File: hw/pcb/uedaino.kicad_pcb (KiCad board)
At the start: 2 copper layers, 34 parts, among them IC1 ATMEGA328P-A, P1 CN_PWR, P2 CN_UART, P3 CN_HEADER1, P4 CN_I2C, P5 CN_HEADER2, P6 CN_ICSP, SW1 SW_PUSH, U1 AP1117, Y1 16MHz

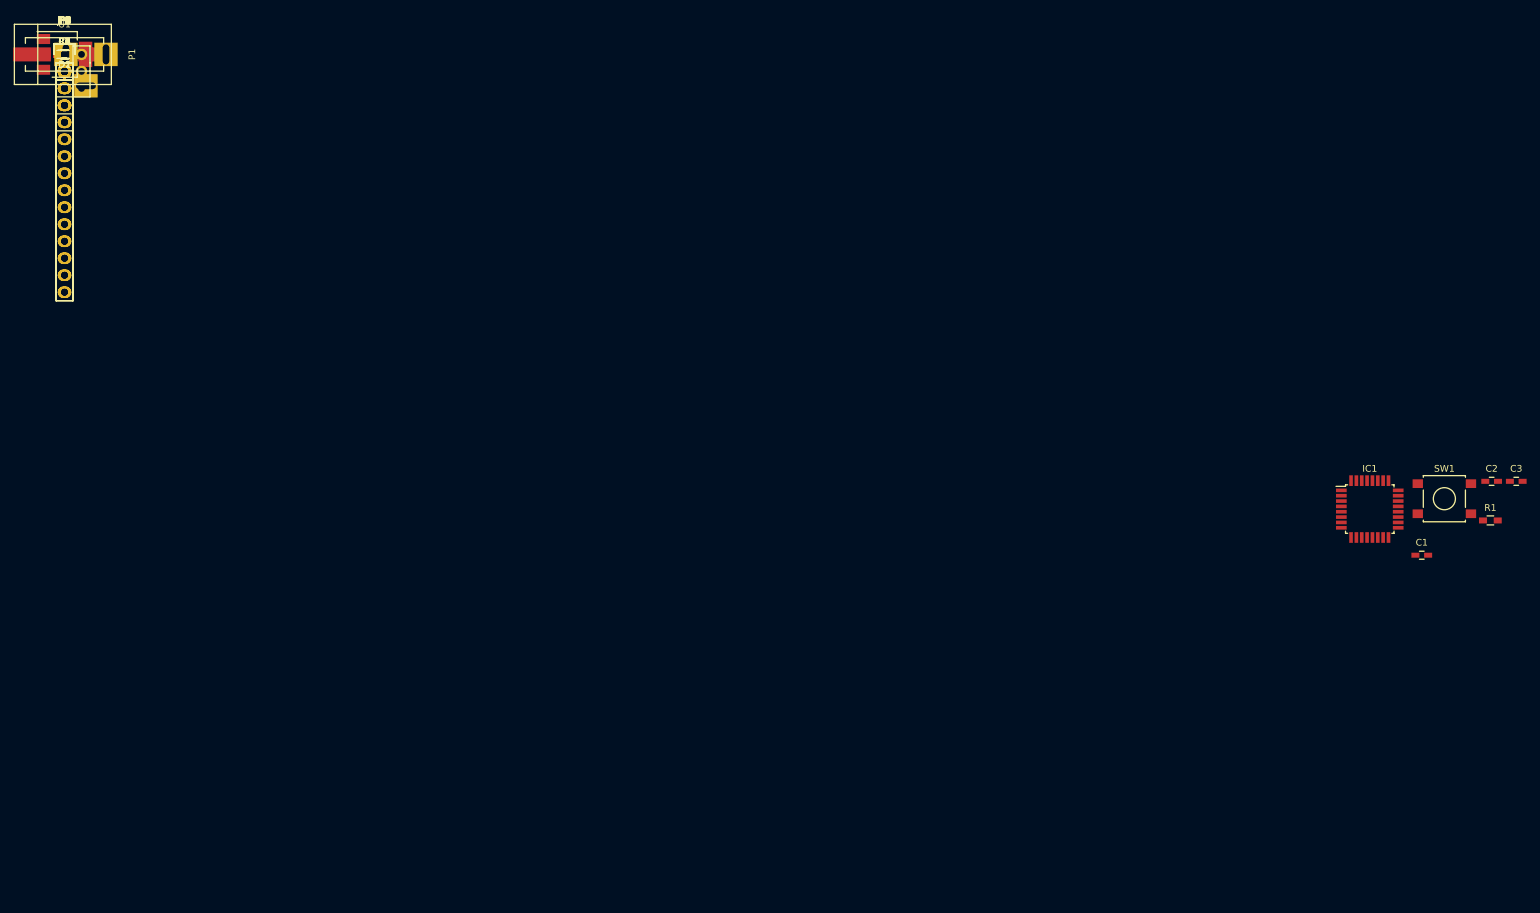
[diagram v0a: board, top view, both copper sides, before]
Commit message: Add PCB Design
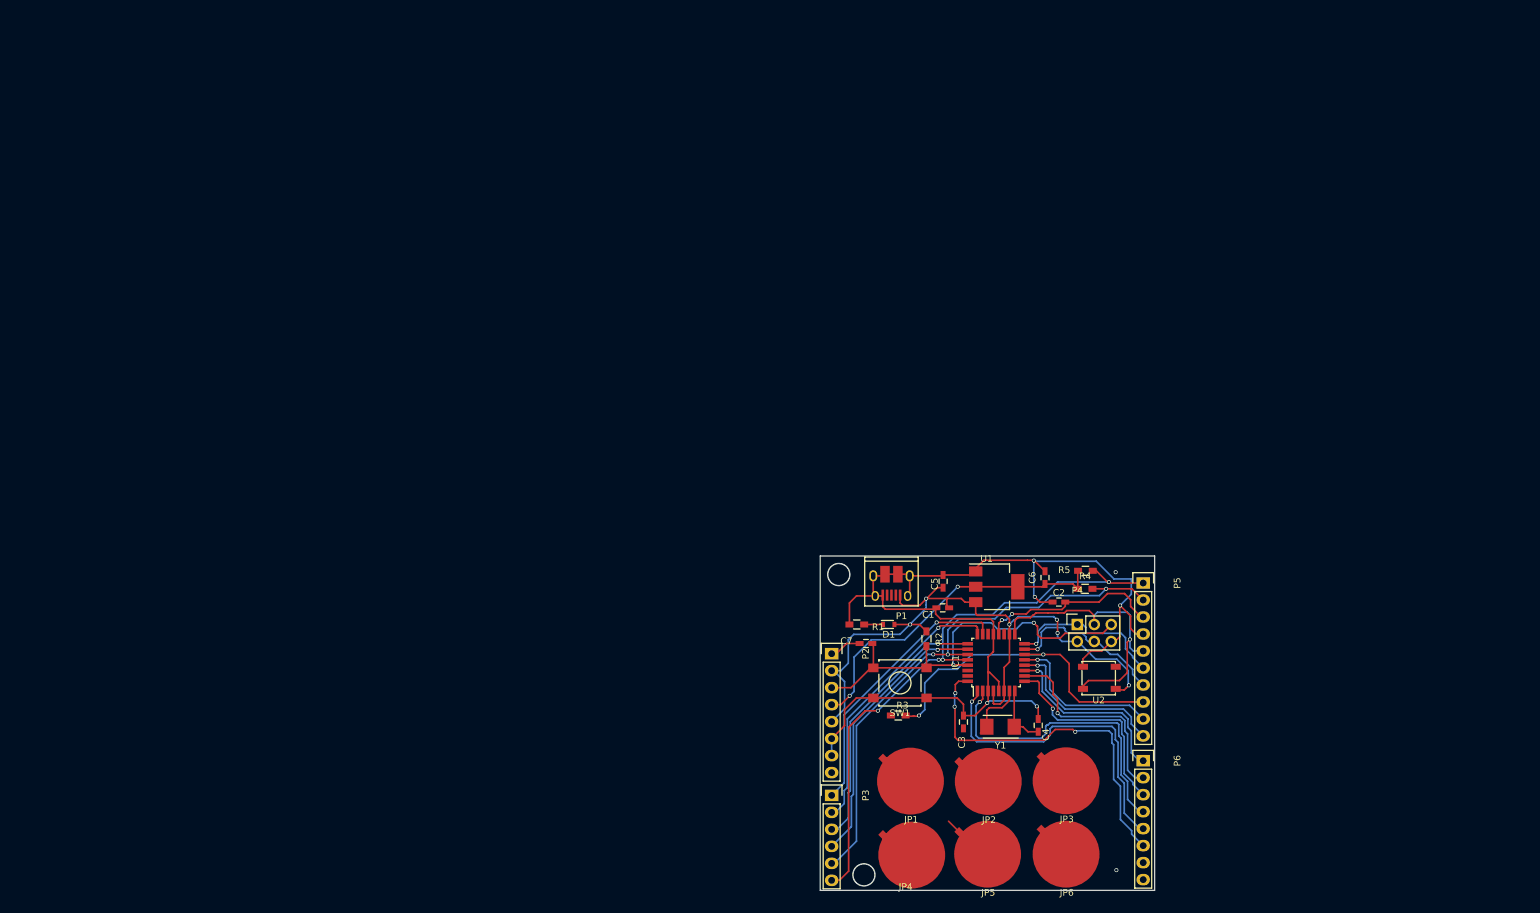
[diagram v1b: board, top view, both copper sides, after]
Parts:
- removed D2: LED_+3V3, Diodes_SMD:D_0603
- removed JP7, JP8, JP9: Jumper_NC_Small, Pin_Headers:Pin_Header_Straight_1x02
- removed R6: 4.7K, Resistors_SMD:R_0603_HandSoldering
- added U2: WS2812B, UeduinoLib:WS2812B, F.Cu at (154.6, 93.3)
- C3: value 0.1u -> 22uF
- C4: value 10uF -> 22uF
- C6: value 22uF -> 10uF
- C7: value 22uF -> 0.1u
- JP1: value Jumper_NC_Small -> J_CAP1; footprint Pin_Headers:Pin_Header_Straight_1x02 -> UeduinoLib:JP_CAP
- JP2: value Jumper_NC_Small -> J_CAP2; footprint Pin_Headers:Pin_Header_Straight_1x02 -> UeduinoLib:JP_CAP
- JP3: value Jumper_NC_Small -> J_CAP3; footprint Pin_Headers:Pin_Header_Straight_1x02 -> UeduinoLib:JP_CAP
- JP4: value Jumper_NC_Small -> J_CAP4; footprint Pin_Headers:Pin_Header_Straight_1x02 -> UeduinoLib:JP_CAP
- JP5: value Jumper_NC_Small -> J_CAP5; footprint Pin_Headers:Pin_Header_Straight_1x02 -> UeduinoLib:JP_CAP
- JP6: value Jumper_NC_Small -> J_CAP6; footprint Pin_Headers:Pin_Header_Straight_1x02 -> UeduinoLib:JP_CAP
- P1: value CN_PWR -> USB_OTG; footprint Connect:BARREL_JACK -> Connectors:USB_Micro-B_10103594-0001LF
- P2: value CN_UART -> CN_POWER; footprint Pin_Headers:Pin_Header_Straight_1x05 -> Socket_Strips:Socket_Strip_Straight_1x08
- P3: value CN_HEADER1 -> CN_J1; footprint Pin_Headers:Pin_Header_Straight_1x15 -> Socket_Strips:Socket_Strip_Straight_1x06
- P4: value CN_I2C -> CN_ICSP; footprint Pin_Headers:Pin_Header_Straight_1x04 -> Socket_Strips:Socket_Strip_Straight_2x03
- P5: value CN_HEADER2 -> CONN_01X10; footprint Pin_Headers:Pin_Header_Straight_1x15 -> Socket_Strips:Socket_Strip_Straight_1x10
- P6: value CN_ICSP -> CONN_01X08; footprint Pin_Headers:Pin_Header_Straight_2x03 -> Socket_Strips:Socket_Strip_Straight_1x08
- R1: value 10K -> 1K
- R2: value 10M -> 10K
- R3: value 1K -> 10M
- R4: value 1K -> 3.3K
- R5: value 4.7K -> 3.3K
- Y1: footprint Crystals:Crystal_HC49-SD_SMD -> Crystals:Crystal_SMD_5032_2Pads
- moved P6 192.8 mm to (161.3, 105.6), turned to 270 degrees
- moved JP6 191.6 mm to (149.8, 119.6)
- moved JP3 185.0 mm to (149.8, 108.6)
- moved JP5 182.6 mm to (138.0, 119.6)
- moved P5 179.6 mm to (161.3, 79.0), turned to 270 degrees
- moved C4 176.8 mm to (145.6, 100.3), turned to 270 degrees
- moved JP2 175.8 mm to (138.1, 108.7)
- moved P4 173.8 mm to (151.4, 85.2)
- moved JP4 172.9 mm to (125.7, 118.7)
- moved Y1 172.3 mm to (140.0, 100.5), turned to 180 degrees
- moved R4 172.3 mm to (152.6, 79.9)
- moved R5 171.1 mm to (152.7, 77.2)
- moved JP1 166.8 mm to (126.5, 108.7)
- moved C6 166.2 mm to (146.6, 78.2), turned to 90 degrees
- moved U1 160.5 mm to (139.4, 79.6)
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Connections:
- C2 pad 1: Net-(C2-Pad1) -> /AREF
- C3 pad 1: /DTR -> /XT1
- C3 pad 2: /RESET -> GND
- C4 pad 1: +5V -> GND
- C4 pad 2: GND -> /XT2
- C5 pad 1: +3V3 -> +5V
- C6 pad 1: /XT1 -> +3V3
- C7 pad 1: GND -> /DTR
- C7 pad 2: /XT2 -> /RESET
- IC1 pad 15: /D11 -> /D11/MOSI
- IC1 pad 16: /D12 -> /D12/MISO
- IC1 pad 17: /D13 -> /D13/SCK
- IC1 pad 19: /A6 -> (no net)
- IC1 pad 20: Net-(C2-Pad1) -> /AREF
- IC1 pad 22: /A7 -> (no net)
- JP1 pad 1: /D13 -> /D9
- JP2 pad 1: Net-(JP2-Pad1) -> /D8
- JP2 pad 2: /D12 -> Net-(JP1-Pad2)
- JP3 pad 1: Net-(JP2-Pad1) -> /D7
- JP3 pad 2: /D11 -> Net-(JP1-Pad2)
- JP4 pad 1: Net-(JP2-Pad1) -> /D6
- JP4 pad 2: /D10 -> Net-(JP1-Pad2)
- JP5 pad 1: Net-(JP2-Pad1) -> /D5
- JP5 pad 2: /D9 -> Net-(JP1-Pad2)
- JP6 pad 1: Net-(JP2-Pad1) -> /D4
- JP6 pad 2: /D8 -> Net-(JP1-Pad2)
- P1 pad 1: (no net) -> +5V
- P1 pad 2: GND -> (no net)
- P2 pad 1: /RXD -> /DTR
- P2 pad 2: /TXD -> +5V
- P2 pad 3: (no net) -> /RESET
- P2 pad 4: GND -> +3V3
- P2 pad 5: /DTR -> +5V
- P3 pad 1: /TXD -> /A0
- P3 pad 2: /RXD -> /A1
- P3 pad 3: /RESET -> /A2
- P3 pad 4: GND -> /A3
- P3 pad 5: /D2 -> /A4/SDA
- P3 pad 6: /D3 -> /A5/SCL
- P4 pad 1: +3V3 -> /D12/MISO
- P4 pad 2: Net-(JP8-Pad2) -> +5V
- P4 pad 3: Net-(JP9-Pad1) -> /D13/SCK
- P4 pad 4: GND -> /D11/MOSI
- P5 pad 1: (no net) -> /A5/SCL
- P5 pad 10: /A2 -> /D8
- P5 pad 2: GND -> /A4/SDA
- P5 pad 3: /RESET -> /AREF
- P5 pad 4: +5V -> GND
- P5 pad 5: /A7 -> /D13/SCK
- P5 pad 6: /A6 -> /D12/MISO
- P5 pad 7: /A5/SCL -> /D11/MOSI
- P5 pad 8: /A4/SDA -> /D10
- P5 pad 9: /A3 -> /D9
- P6 pad 1: /D12 -> /D7
- P6 pad 2: +5V -> /D6
- P6 pad 3: /D13 -> /D5
- P6 pad 4: /D11 -> /D4
- P6 pad 5: /RESET -> /D3
- P6 pad 6: GND -> /D2
- R1 pad 1: +5V -> Net-(D1-Pad1)
- R1 pad 2: /RESET -> GND
- R2 pad 1: Net-(JP1-Pad2) -> +5V
- R2 pad 2: Net-(JP2-Pad1) -> /RESET
- R3 pad 1: Net-(D1-Pad1) -> /D10
- R3 pad 2: GND -> Net-(JP1-Pad2)
- R4 pad 1: Net-(D2-Pad1) -> +3V3
- R4 pad 2: GND -> /A4/SDA
- R5 pad 2: Net-(JP9-Pad1) -> /A5/SCL
- U1 pad 4: (no net) -> +3V3
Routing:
- net GND: track 0.00 -> 170.3 mm, vias 0 -> 5
- net +5V: track 0.00 -> 105.8 mm, vias 0 -> 6
- net /A5/SCL: track 0.00 -> 87.4 mm, vias 0 -> 4
- net /A4/SDA: track 0.00 -> 81.6 mm, vias 0 -> 3
- net /RESET: track 0.00 -> 63.4 mm, vias 0 -> 2
- net /D2: track 0.00 -> 53.4 mm, vias 0 -> 3
- net /D10: track 0.00 -> 50.8 mm, vias 0 -> 2
- net +3V3: track 0.00 -> 50.3 mm, vias 0 -> 2
- net /D3: track 0.00 -> 47.6 mm, vias 0 -> 1
- net /D4: track 0.00 -> 45.6 mm, vias 0 -> 1
- net /D13/SCK: track 0.00 -> 43.3 mm, vias 0 -> 1
- net /A1: track 0.00 -> 41.6 mm, vias 0 -> 1
- net /A3: track 0.00 -> 41.5 mm, vias 0 -> 1
- net /A2: track 0.00 -> 41.1 mm, vias 0 -> 1
- net /A0: track 0.00 -> 40.9 mm, vias 0 -> 1
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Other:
- board outline added: 50 x 50 mm
- net class Power added: clearance 0.2, trace_width 1, via_dia 0.6, via_drill 0.4
